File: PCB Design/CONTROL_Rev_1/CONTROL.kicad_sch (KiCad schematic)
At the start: 50 parts, among them J1 Conn_01x24_Pin, J2 Conn_01x24_Pin, J3 Micro_SD_Card, J4 USB_C_Receptacle_USB2.0_16P, SW1 SW_SPDT, U1 STM32F446RET6, U2 USBLC6-2SC6, Y1 16MHz, Y2 32.768KHz

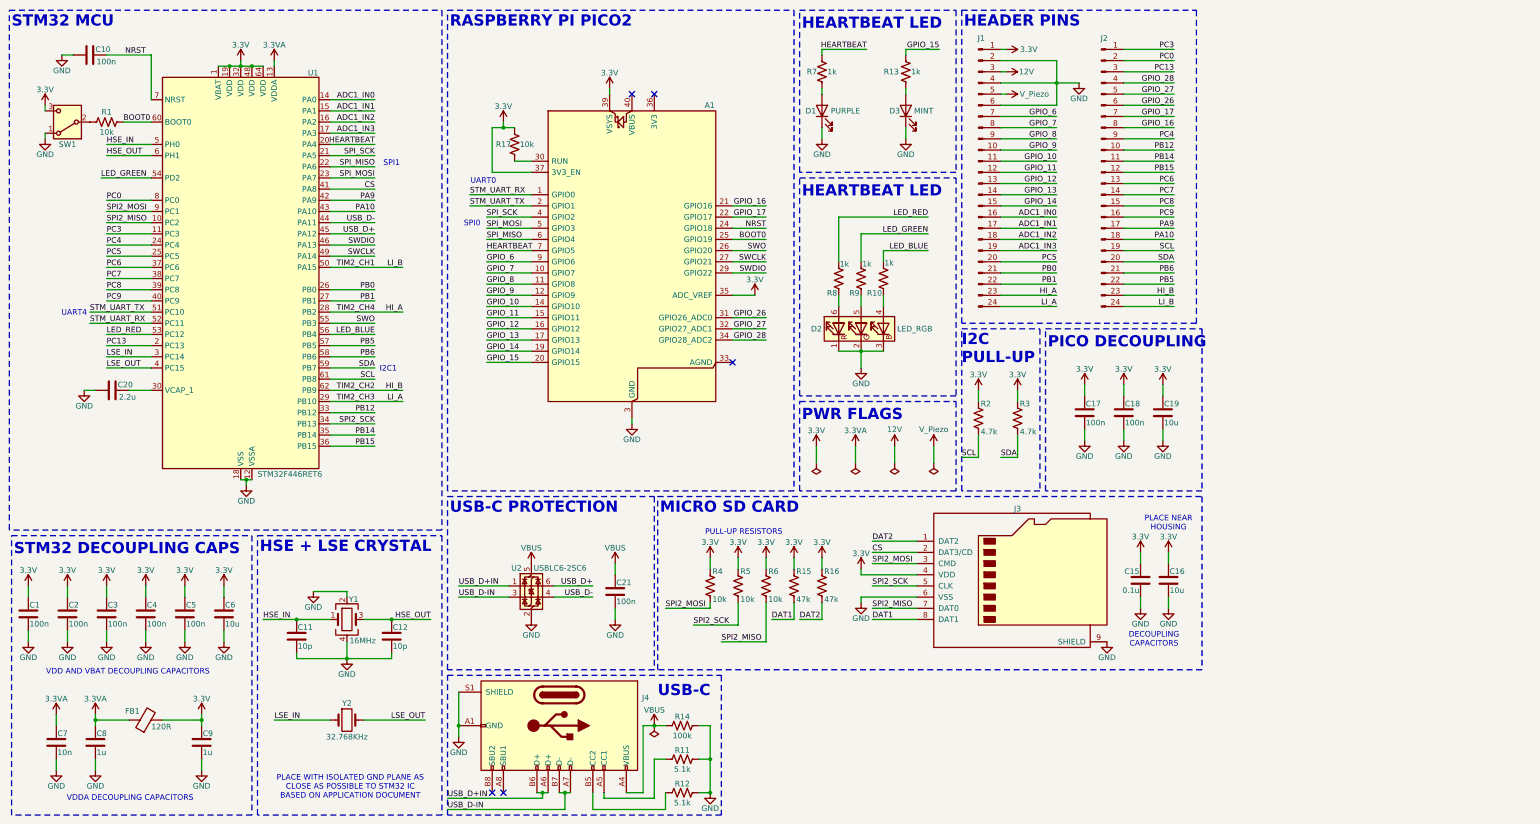
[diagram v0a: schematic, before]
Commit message: Updated
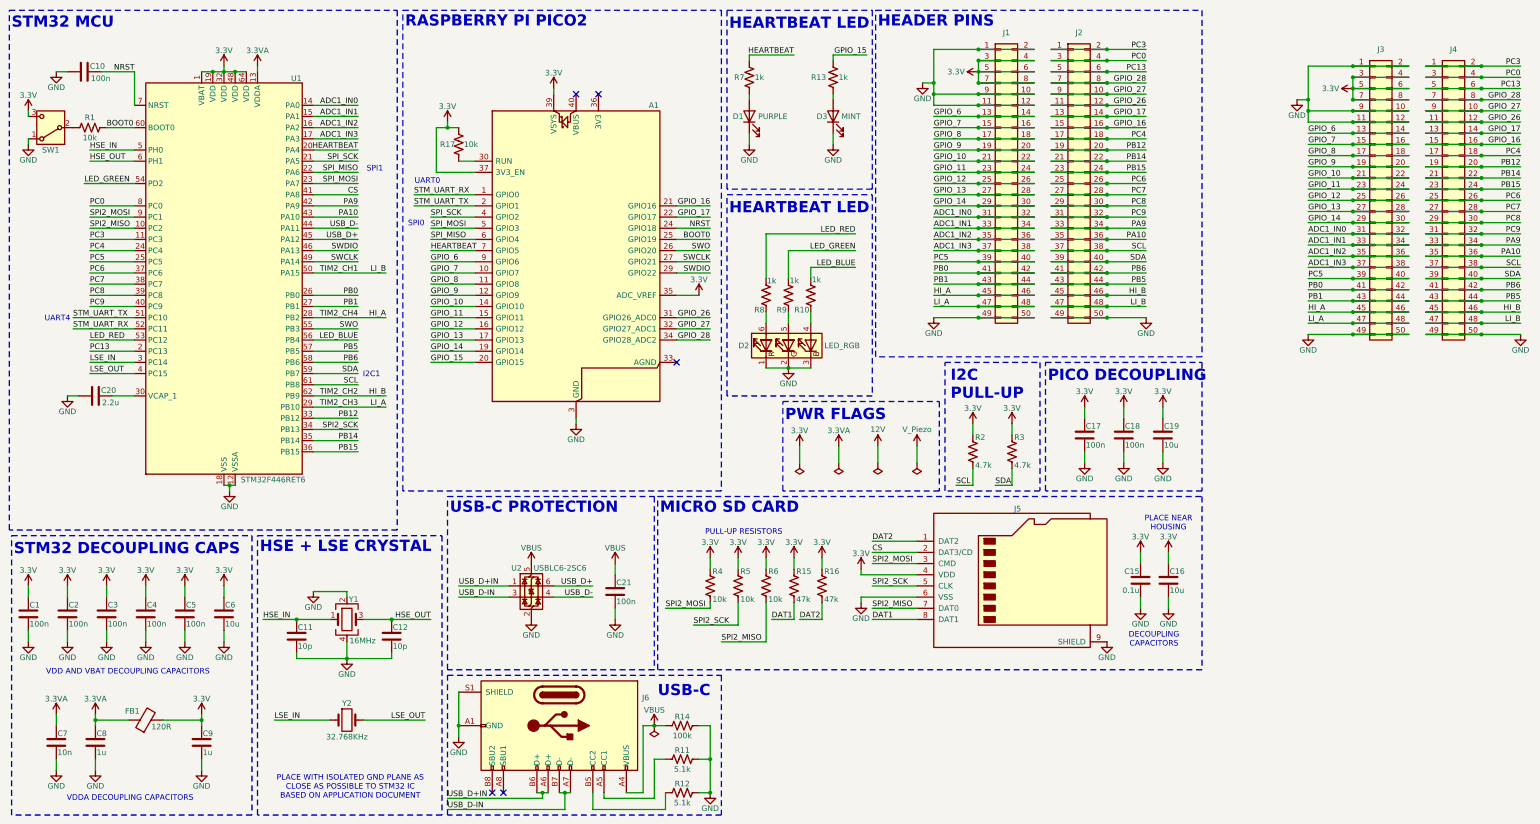
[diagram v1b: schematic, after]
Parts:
- removed J1, J2: Conn_01x24_Pin, Connector_PinHeader_2.54mm:PinHeader_1x24_P2.54mm_Vertical, symbol Connector:Conn_01x24_Pin
- added J1, J2, J3, J4: Conn_02x25_Odd_Even, CONTROL:HIROSE_DF40C-50DP-0.4V_51_, symbol Connector_Generic:Conn_02x25_Odd_Even
- renumbered J3 to J5, J4 to J6
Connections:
- net 3.3V: now also J1.3 (Pin_3), J1.4 (Pin_4), J1.5 (Pin_5), J1.6 (Pin_6), J1.7 (Pin_7), J1.8 (Pin_8), J3.3 (Pin_3), J3.4 (Pin_4), J3.5 (Pin_5), J3.6 (Pin_6), J3.7 (Pin_7), J3.8 (Pin_8)
- net ADC1_IN0: now also J1.31 (Pin_31), J1.32 (Pin_32), J3.31 (Pin_31), J3.32 (Pin_32)
- net ADC1_IN1: now also J1.33 (Pin_33), J1.34 (Pin_34), J3.33 (Pin_33), J3.34 (Pin_34)
- net ADC1_IN2: now also J1.35 (Pin_35), J1.36 (Pin_36), J3.35 (Pin_35), J3.36 (Pin_36)
- net ADC1_IN3: now also J1.37 (Pin_37), J1.38 (Pin_38), J3.37 (Pin_37), J3.38 (Pin_38)
- net GND: now also J1.1 (Pin_1), J1.10 (Pin_10), J1.11 (Pin_11), J1.12 (Pin_12), J1.2 (Pin_2), J1.49 (Pin_49), J1.50 (Pin_50), J1.9 (Pin_9), J2.49 (Pin_49), J2.50 (Pin_50), J3.1 (Pin_1), J3.10 (Pin_10), J3.11 (Pin_11), J3.12 (Pin_12), J3.2 (Pin_2), J3.49 (Pin_49), J3.50 (Pin_50), J3.9 (Pin_9), J4.49 (Pin_49), J4.50 (Pin_50)
- net GPIO_10: now also J1.21 (Pin_21), J1.22 (Pin_22), J3.21 (Pin_21), J3.22 (Pin_22)
- net GPIO_11: now also J1.23 (Pin_23), J1.24 (Pin_24), J3.23 (Pin_23), J3.24 (Pin_24)
- net GPIO_12: now also J1.25 (Pin_25), J1.26 (Pin_26), J3.25 (Pin_25), J3.26 (Pin_26)
- net GPIO_13: now also J1.27 (Pin_27), J1.28 (Pin_28), J3.27 (Pin_27), J3.28 (Pin_28)
- net GPIO_14: now also J1.29 (Pin_29), J1.30 (Pin_30), J3.29 (Pin_29), J3.30 (Pin_30)
- net GPIO_16: now also J2.15 (Pin_15), J2.16 (Pin_16), J4.15 (Pin_15), J4.16 (Pin_16)
- net GPIO_17: now also J2.13 (Pin_13), J2.14 (Pin_14), J4.13 (Pin_13), J4.14 (Pin_14)
- net GPIO_26: now also J2.11 (Pin_11), J2.12 (Pin_12), J4.11 (Pin_11), J4.12 (Pin_12)
- net GPIO_27: now also J2.10 (Pin_10), J2.9 (Pin_9), J4.10 (Pin_10), J4.9 (Pin_9)
- net GPIO_28: now also J2.7 (Pin_7), J2.8 (Pin_8), J4.7 (Pin_7), J4.8 (Pin_8)
- net GPIO_6: now also J1.13 (Pin_13), J1.14 (Pin_14), J3.13 (Pin_13), J3.14 (Pin_14)
- net GPIO_7: now also J1.15 (Pin_15), J1.16 (Pin_16), J3.15 (Pin_15), J3.16 (Pin_16)
- net GPIO_8: now also J1.17 (Pin_17), J1.18 (Pin_18), J3.17 (Pin_17), J3.18 (Pin_18)
- net GPIO_9: now also J1.19 (Pin_19), J1.20 (Pin_20), J3.19 (Pin_19), J3.20 (Pin_20)
- net HI_A: now also J1.45 (Pin_45), J1.46 (Pin_46), J3.45 (Pin_45), J3.46 (Pin_46)
- net HI_B: now also J2.45 (Pin_45), J2.46 (Pin_46), J4.45 (Pin_45), J4.46 (Pin_46)
- net LI_A: now also J1.47 (Pin_47), J1.48 (Pin_48), J3.47 (Pin_47), J3.48 (Pin_48)
- net LI_B: now also J2.47 (Pin_47), J2.48 (Pin_48), J4.47 (Pin_47), J4.48 (Pin_48)
- net PA10: now also J2.35 (Pin_35), J2.36 (Pin_36), J4.35 (Pin_35), J4.36 (Pin_36)
- net PA9: now also J2.33 (Pin_33), J2.34 (Pin_34), J4.33 (Pin_33), J4.34 (Pin_34)
- net PB0: now also J1.41 (Pin_41), J1.42 (Pin_42), J3.41 (Pin_41), J3.42 (Pin_42)
- net PB1: now also J1.43 (Pin_43), J1.44 (Pin_44), J3.43 (Pin_43), J3.44 (Pin_44)
- net PB12: now also J2.19 (Pin_19), J2.20 (Pin_20), J4.19 (Pin_19), J4.20 (Pin_20)
- net PB14: now also J2.21 (Pin_21), J2.22 (Pin_22), J4.21 (Pin_21), J4.22 (Pin_22)
- net PB15: now also J2.23 (Pin_23), J2.24 (Pin_24), J4.23 (Pin_23), J4.24 (Pin_24)
- net PB5: now also J2.43 (Pin_43), J2.44 (Pin_44), J4.43 (Pin_43), J4.44 (Pin_44)
- net PB6: now also J2.41 (Pin_41), J2.42 (Pin_42), J4.41 (Pin_41), J4.42 (Pin_42)
- net PC0: now also J2.3 (Pin_3), J2.4 (Pin_4), J4.3 (Pin_3), J4.4 (Pin_4)
- net PC13: now also J2.5 (Pin_5), J2.6 (Pin_6), J4.5 (Pin_5), J4.6 (Pin_6)
- net PC3: now also J2.1 (Pin_1), J2.2 (Pin_2), J4.1 (Pin_1), J4.2 (Pin_2)
- net PC4: now also J2.17 (Pin_17), J2.18 (Pin_18), J4.17 (Pin_17), J4.18 (Pin_18)
- net PC5: now also J1.39 (Pin_39), J1.40 (Pin_40), J3.39 (Pin_39), J3.40 (Pin_40)
- net PC6: now also J2.25 (Pin_25), J2.26 (Pin_26), J4.25 (Pin_25), J4.26 (Pin_26)
- net PC7: now also J2.27 (Pin_27), J2.28 (Pin_28), J4.27 (Pin_27), J4.28 (Pin_28)
- net PC8: now also J2.29 (Pin_29), J2.30 (Pin_30), J4.29 (Pin_29), J4.30 (Pin_30)
- net PC9: now also J2.31 (Pin_31), J2.32 (Pin_32), J4.31 (Pin_31), J4.32 (Pin_32)
- net SCL: now also J2.37 (Pin_37), J2.38 (Pin_38), J4.37 (Pin_37), J4.38 (Pin_38)
- net SDA: now also J2.39 (Pin_39), J2.40 (Pin_40), J4.39 (Pin_39), J4.40 (Pin_40)
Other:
- moved on the sheet: A1, C10, C17, C18, C19, C20, D1, D2, D3, R1, R10, R13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

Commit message: Revert "Updated"
This reverts commit 89be44ed720659141c8ee702c54a520a60db740f.
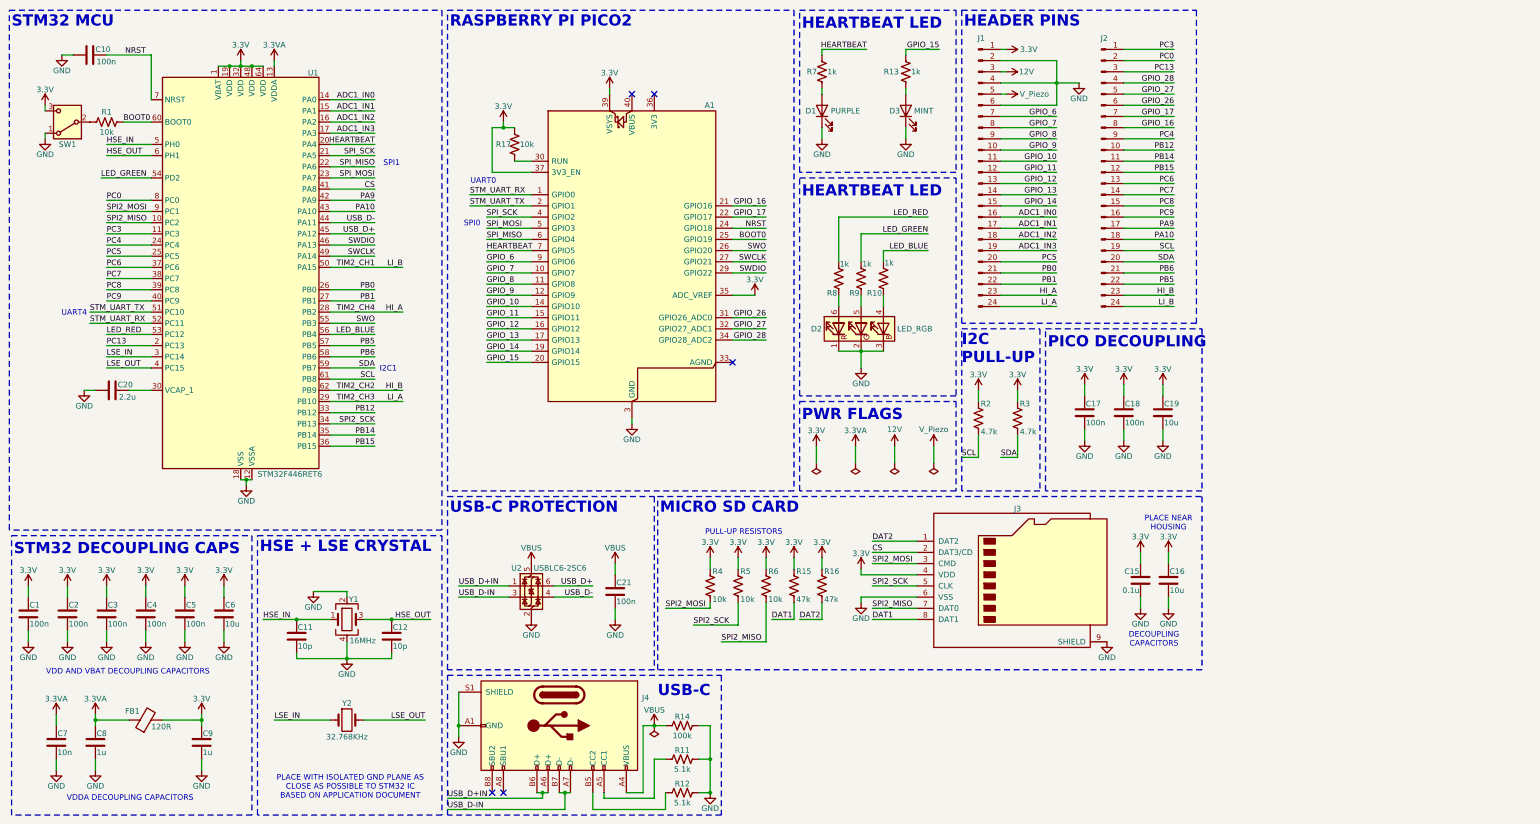
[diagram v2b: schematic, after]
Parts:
- removed J1, J2, J3, J4: Conn_02x25_Odd_Even, CONTROL:HIROSE_DF40C-50DP-0.4V_51_, symbol Connector_Generic:Conn_02x25_Odd_Even
- added J1, J2: Conn_01x24_Pin, Connector_PinHeader_2.54mm:PinHeader_1x24_P2.54mm_Vertical, symbol Connector:Conn_01x24_Pin
- renumbered J5 to J3, J6 to J4
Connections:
- net 12V: now also J1.3 (Pin_3)
- net 3.3V: now also J1.1 (Pin_1)
- net ADC1_IN0: now also J1.16 (Pin_16)
- net ADC1_IN1: now also J1.17 (Pin_17)
- net ADC1_IN2: now also J1.18 (Pin_18)
- net ADC1_IN3: now also J1.19 (Pin_19)
- net GND: now also J1.2 (Pin_2), J1.4 (Pin_4), J1.6 (Pin_6)
- net GPIO_10: now also J1.11 (Pin_11)
- net GPIO_11: now also J1.12 (Pin_12)
- net GPIO_12: now also J1.13 (Pin_13)
- net GPIO_13: now also J1.14 (Pin_14)
- net GPIO_14: now also J1.15 (Pin_15)
- net GPIO_16: now also J2.8 (Pin_8)
- net GPIO_17: now also J2.7 (Pin_7)
- net GPIO_26: now also J2.6 (Pin_6)
- net GPIO_27: now also J2.5 (Pin_5)
- net GPIO_28: now also J2.4 (Pin_4)
- net GPIO_6: now also J1.7 (Pin_7)
- net GPIO_7: now also J1.8 (Pin_8)
- net GPIO_8: now also J1.9 (Pin_9)
- net GPIO_9: now also J1.10 (Pin_10)
- net HI_A: now also J1.23 (Pin_23)
- net HI_B: now also J2.23 (Pin_23)
- net LI_A: now also J1.24 (Pin_24)
- net LI_B: now also J2.24 (Pin_24)
- net PA10: now also J2.18 (Pin_18)
- net PA9: now also J2.17 (Pin_17)
- net PB0: now also J1.21 (Pin_21)
- net PB1: now also J1.22 (Pin_22)
- net PB12: now also J2.10 (Pin_10)
- net PB14: now also J2.11 (Pin_11)
- net PB15: now also J2.12 (Pin_12)
- net PB5: now also J2.22 (Pin_22)
- net PB6: now also J2.21 (Pin_21)
- net PC0: now also J2.2 (Pin_2)
- net PC13: now also J2.3 (Pin_3)
- net PC3: now also J2.1 (Pin_1)
- net PC4: now also J2.9 (Pin_9)
- net PC5: now also J1.20 (Pin_20)
- net PC6: now also J2.13 (Pin_13)
- net PC7: now also J2.14 (Pin_14)
- net PC8: now also J2.15 (Pin_15)
- net PC9: now also J2.16 (Pin_16)
- net SCL: now also J2.19 (Pin_19)
- net SDA: now also J2.20 (Pin_20)
- net V_Piezo: now also J1.5 (Pin_5)
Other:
- moved on the sheet: A1, C10, C17, C18, C19, C20, D1, D2, D3, R1, R10, R13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
